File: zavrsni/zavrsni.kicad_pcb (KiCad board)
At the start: 2 copper layers, 228.6 x 139.7 mm, 63 parts, among them Q1 BC337, Q2 BC317, SW1 EC11_SW, U1 CS4335, U2 WeAct STM32F411CEU6 v3.0, U3 NE5532, U4 TL074, U5 LM358, U6 LM317_TO-220, U7 UC1609C LCD Board

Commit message: PCB is done
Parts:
- removed SW1: EC11_SW, ljepi:ec11
- removed SW_PRESET_7: SW_Push, Button_Switch_THT:SW_PUSH_6mm_H13mm
- U6: footprint Package_TO_SOT_THT:TO-220-3_Vertical -> Package_TO_SOT_THT:TO-220-3_Horizontal_TabDown
- moved C9 190.9 mm to (56.7, 101.4), turned to -90 degrees
- moved SW_UP1 173.0 mm to (184.4, 98.0), turned to 90 degrees
- moved SW_DOWN1 168.8 mm to (184.4, 113.0), turned to 90 degrees
- moved C13 165.2 mm to (107.5, 93.9), turned to 90 degrees
- moved U1 155.1 mm to (115.1, 60.5), turned to 90 degrees
- moved SW_OK1 154.5 mm to (184.4, 72.0), turned to 90 degrees
- moved C4 151.6 mm to (106.5, 62.4), turned to 90 degrees
- moved C12 150.6 mm to (104.2, 88.4)
- moved C3 144.0 mm to (110.8, 62.2), turned to 90 degrees
- moved SW_PRESET_3 135.7 mm to (184.7, 134.8), turned to 90 degrees
- moved SW_PRESET_2 125.2 mm to (162.1, 134.8), turned to 90 degrees
- moved SW_PRESET_0 124.1 mm to (102.1, 134.8), turned to 90 degrees
- moved Jout1 123.1 mm to (120.2, 57.9)
- moved SW_PRESET_1 118.4 mm to (132.1, 134.8), turned to 90 degrees
- moved Jvss1 97.5 mm to (55.0, 135.3), turned to -90 degrees
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- renumbered SW_PRESET_5 to SW_DOWN1, SW_PRESET_6 to SW_OK1, SW_PRESET_4 to SW_UP1
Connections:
- net /PRESET0 renamed /BTN_PRESET0
- net /PRESET1 renamed /BTN_PRESET1
- net /PRESET2 renamed /BTN_PRESET2
- net /PRESET3 renamed /BTN_PRESET3
- net /PRESET6 renamed /BTN_OK
- SW_DOWN1 pad 1: /PRESET5 -> /BTN_DOWN
- SW_UP1 pad 1: /PRESET4 -> /BTN_UP
- U2 pad 11: /PRESET5 -> /BTN_UP
- U2 pad 12: /PRESET4 -> /BTN_DOWN
- U2 pad 2: /ROT_B -> /DAC_BCLK
- U2 pad 3: /ROT_A -> unconnected-(U2-B14-Pad3)
- U2 pad 37: /DAC_BCLK -> unconnected-(U2-B10-Pad37)
- U2 pad 38: unconnected-(U2-3V3-Pad38) -> +3V3
- U2 pad 5: /ROT_SW -> unconnected-(U2-A8-Pad5)
- U2 pad 9: /PRESET7 -> unconnected-(U2-A12-Pad9)
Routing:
- net /BTN_PRESET3: track 0.00 -> 145.4 mm
- net /BTN_PRESET2: track 0.00 -> 125.7 mm
- net /BTN_DOWN: track 0.00 -> 117.2 mm
- net /BTN_PRESET0: track 0.00 -> 115.8 mm
- net /BTN_UP: track 0.00 -> 108.2 mm
- net /BTN_PRESET1: track 0.00 -> 99.3 mm
- net /BTN_OK: track 0.00 -> 91.8 mm
- net /LCD_SCK: track 0.00 -> 68.2 mm
- net +5V: track 41.8 -> 97.5 mm
- net /LCD_SDA: track 0.00 -> 54.9 mm
- net /DAC_MCLK: track 0.00 -> 46.1 mm, vias 0 -> 1
- net /LCD_RST: track 0.00 -> 35.2 mm, vias 0 -> 2
- net /LCD_CS: track 0.00 -> 34.0 mm
- net /LCD_CD: track 0.00 -> 30.0 mm
- net +12V: track 80.6 -> 107.6 mm
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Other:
- board size 228.6 x 139.7 mm -> 156.4 x 99.2 mm
- board text added: "${CRTAO} Pedala multiefekata za električnu gitaru ${DATUM} v${VERZIJA}"

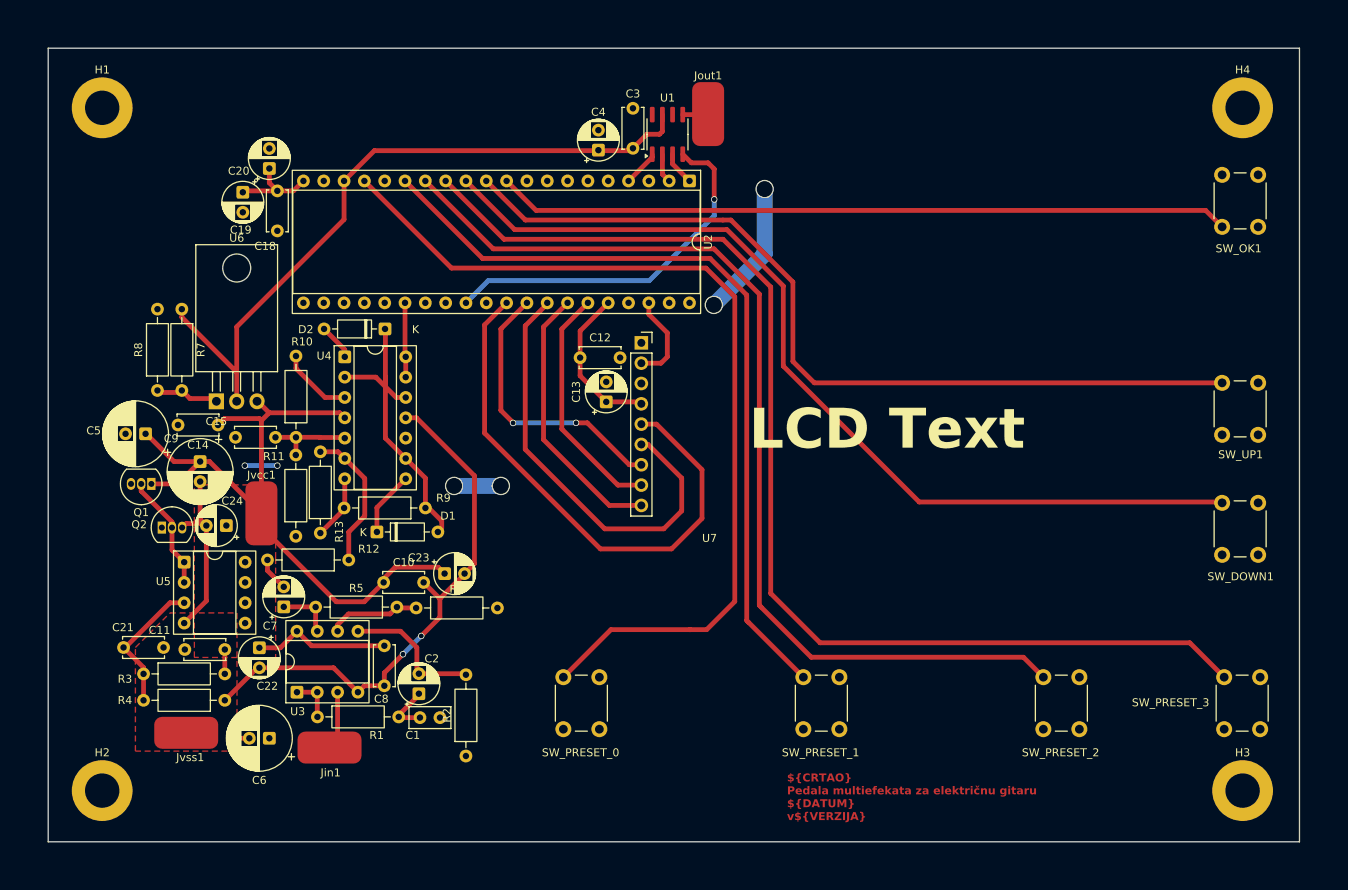
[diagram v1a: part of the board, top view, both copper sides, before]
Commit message: PCB prototype finishing touches
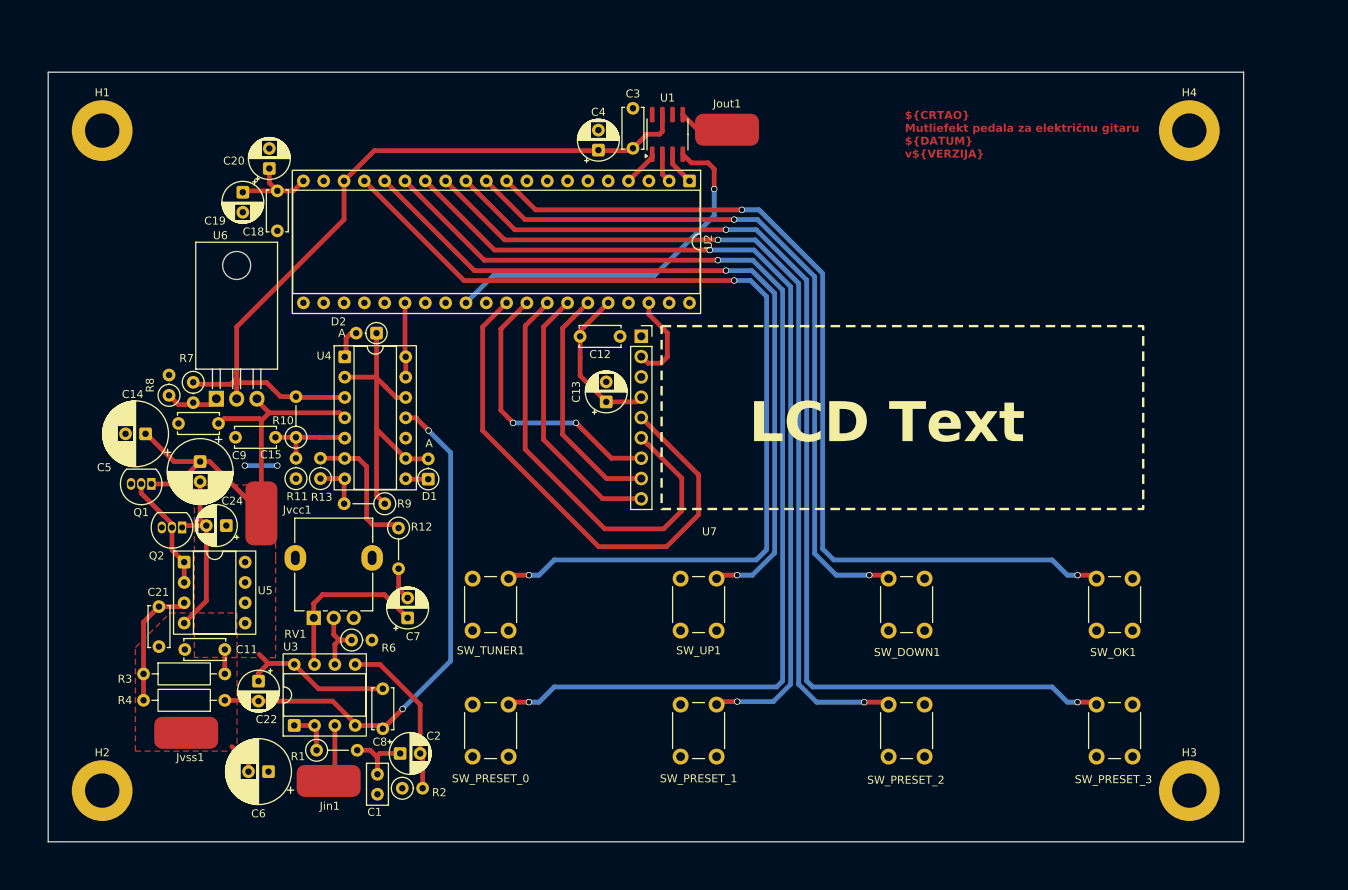
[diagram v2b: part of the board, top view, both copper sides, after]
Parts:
- removed C10: 100n, Capacitor_THT:C_Disc_D5.0mm_W2.5mm_P5.00mm
- removed C23: 10u, Capacitor_THT:CP_Radial_D5.0mm_P2.50mm
- removed R5: 1k, Resistor_THT:R_Axial_DIN0207_L6.3mm_D2.5mm_P10.16mm_Horizontal
- added RV1: R_Potentiometer_MountingPin, ljepi:pot vertikalni 5 pin, F.Cu at (70.9, 120.9)
- added SW_TUNER1: SW_Push, Button_Switch_THT:SW_PUSH_6mm_H13mm, F.Cu at (95.2, 116.0)
- D1, D2: footprint Diode_THT:D_DO-35_SOD27_P7.62mm_Horizontal -> Diode_THT:D_DO-35_SOD27_P2.54mm_Vertical_AnodeUp
- Q2: value BC317 -> BC327
- R1, R10, R12, R9: footprint Resistor_THT:R_Axial_DIN0207_L6.3mm_D2.5mm_P10.16mm_Horizontal -> Resistor_THT:R_Axial_DIN0207_L6.3mm_D2.5mm_P5.08mm_Vertical
- R11, R13, R2, R7, R8: footprint Resistor_THT:R_Axial_DIN0207_L6.3mm_D2.5mm_P10.16mm_Horizontal -> Resistor_THT:R_Axial_DIN0207_L6.3mm_D2.5mm_P2.54mm_Vertical
- R6: value 330 -> 300; footprint Resistor_THT:R_Axial_DIN0207_L6.3mm_D2.5mm_P10.16mm_Horizontal -> Resistor_THT:R_Axial_DIN0207_L6.3mm_D2.5mm_P2.54mm_Vertical
- moved SW_UP1 65.7 mm to (121.2, 116.0), turned to -90 degrees
- moved SW_OK1 52.9 mm to (168.8, 122.5)
- moved SW_DOWN1 42.8 mm to (142.8, 122.5)
- moved SW_PRESET_2 19.6 mm to (142.8, 138.2)
- moved SW_PRESET_3 16.3 mm to (168.8, 138.2)
- moved C7 15.5 mm to (82.6, 120.9)
- moved SW_PRESET_1 11.3 mm to (121.2, 131.8), turned to -90 degrees
- moved R7 9.25 mm to (55.8, 91.5)
- moved D1 9.20 mm to (85.2, 103.6), turned to 90 degrees
- moved R6 9.01 mm to (75.6, 123.7)
- moved R2 8.92 mm to (82.0, 142.2), turned to 0 degrees
- moved C1 8.85 mm to (78.9, 140.5), turned to -90 degrees
- moved C2 7.83 mm to (81.7, 137.9), turned to 0 degrees
- moved SW_PRESET_0 7.50 mm to (95.2, 131.8), turned to -90 degrees
- moved R12 7.39 mm to (81.5, 109.7), turned to -90 degrees
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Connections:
- Q2 pad 1: GNDREF -> +0V
- Q2 pad 3: +0V -> GNDREF
- U2 pad 11: /BTN_UP -> /BTN_DOWN
- U2 pad 12: /BTN_DOWN -> /BTN_PRESET3
- U2 pad 13: /BTN_PRESET3 -> /BTN_PRESET2
- U2 pad 14: /BTN_PRESET2 -> /BTN_PRESET1
- U2 pad 15: /BTN_PRESET1 -> /BTN_PRESET0
- U2 pad 16: unconnected-(U2-B8-Pad16) -> /BTN_UP
- U2 pad 17: /BTN_PRESET0 -> /BTN_TUNER
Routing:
- net /BTN_TUNER: track 0.00 -> 121.6 mm, vias 0 -> 2
- net +12V: track 107.6 -> 79.6 mm
- net /BTN_DOWN: track 117.2 -> 91.1 mm, vias 0 -> 2
- net GNDREF: track 27.0 -> 4.06 mm, vias 6 -> 2
- net /BTN_OK: track 91.8 -> 114.5 mm, vias 0 -> 2
- net /BTN_PRESET0: track 115.8 -> 137.2 mm, vias 0 -> 2
- net Net-(C7-Pad1): track 7.10 -> 21.1 mm
- net /BTN_PRESET2: track 125.7 -> 111.8 mm, vias 0 -> 2
- net /BTN_UP: track 108.2 -> 95.6 mm, vias 0 -> 2
- net /BTN_PRESET1: track 99.3 -> 111.1 mm, vias 0 -> 2
- net /BTN_PRESET3: track 145.4 -> 135.3 mm, vias 0 -> 2
- net Net-(D1-K): track 8.14 -> 2.84 mm
- net Net-(U3B--): track 11.6 -> 7.88 mm
- net Net-(U3B-+): track 17.9 -> 20.8 mm
- net /OUT: track 3.96 -> 6.33 mm
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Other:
- board size 156.4 x 99.2 mm -> 149.4 x 96.2 mm
- board text added: "${CRTAO} Mutliefekt pedala za električnu gitaru ${DATUM} v${VERZIJA}"
- board text removed: "${CRTAO} Pedala multiefekata za električnu gitaru ${DATUM} v${VERZIJA}"
